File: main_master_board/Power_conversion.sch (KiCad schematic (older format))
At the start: 60 parts

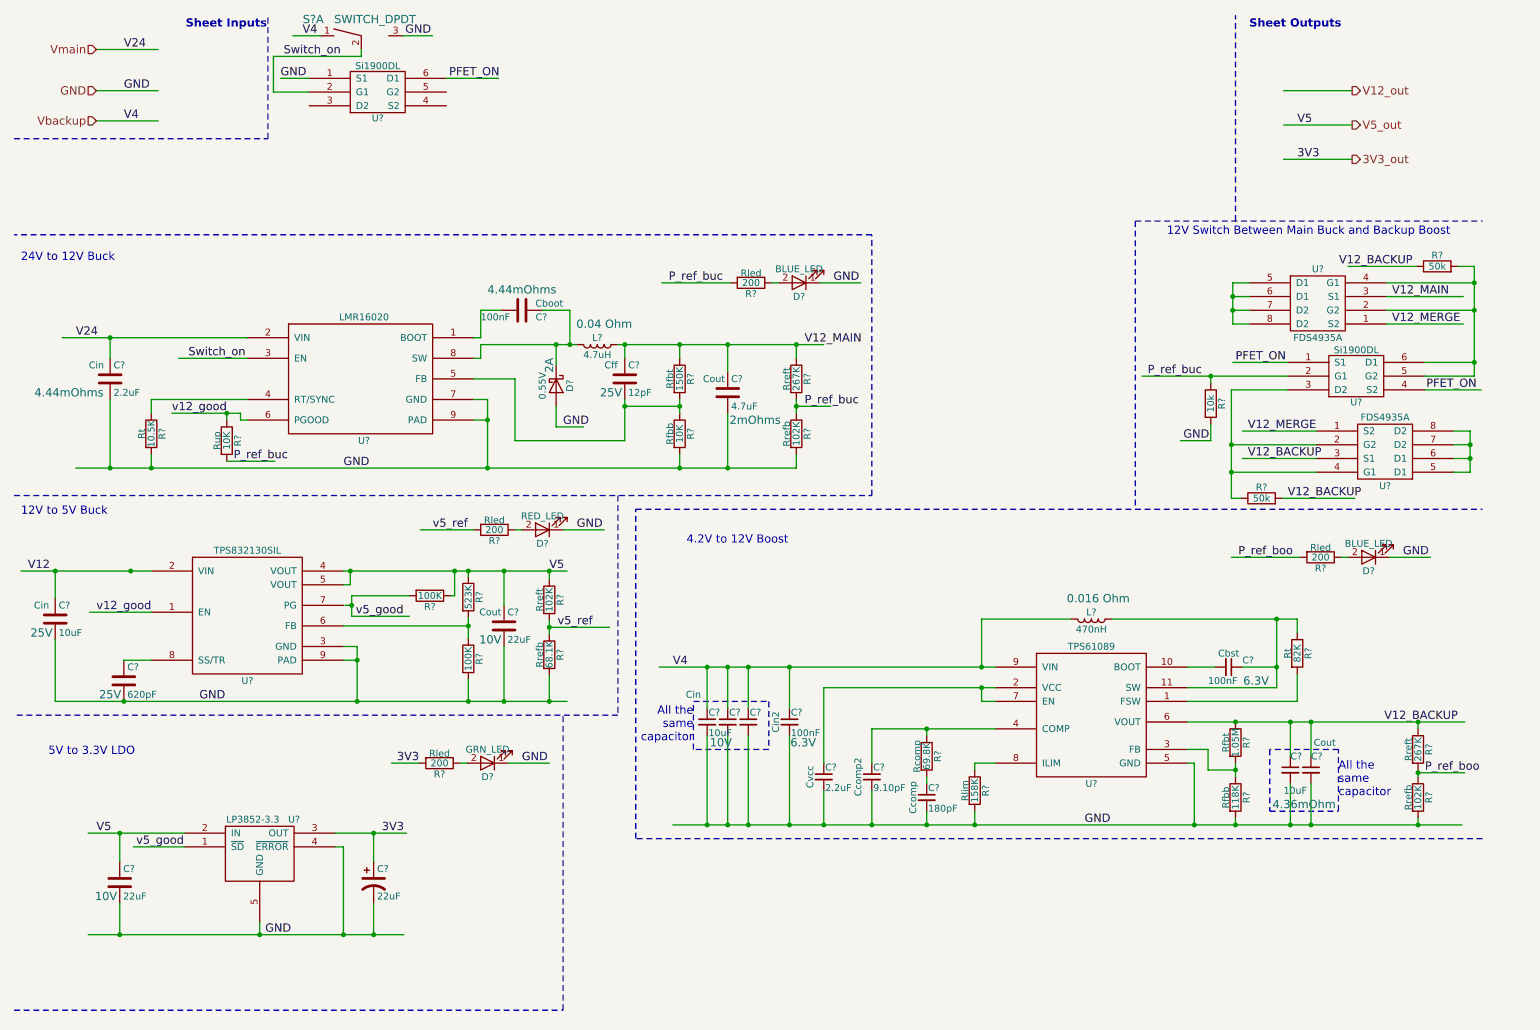
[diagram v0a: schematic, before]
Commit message: Added lots of things. current/voltage monitoring. and other stuff
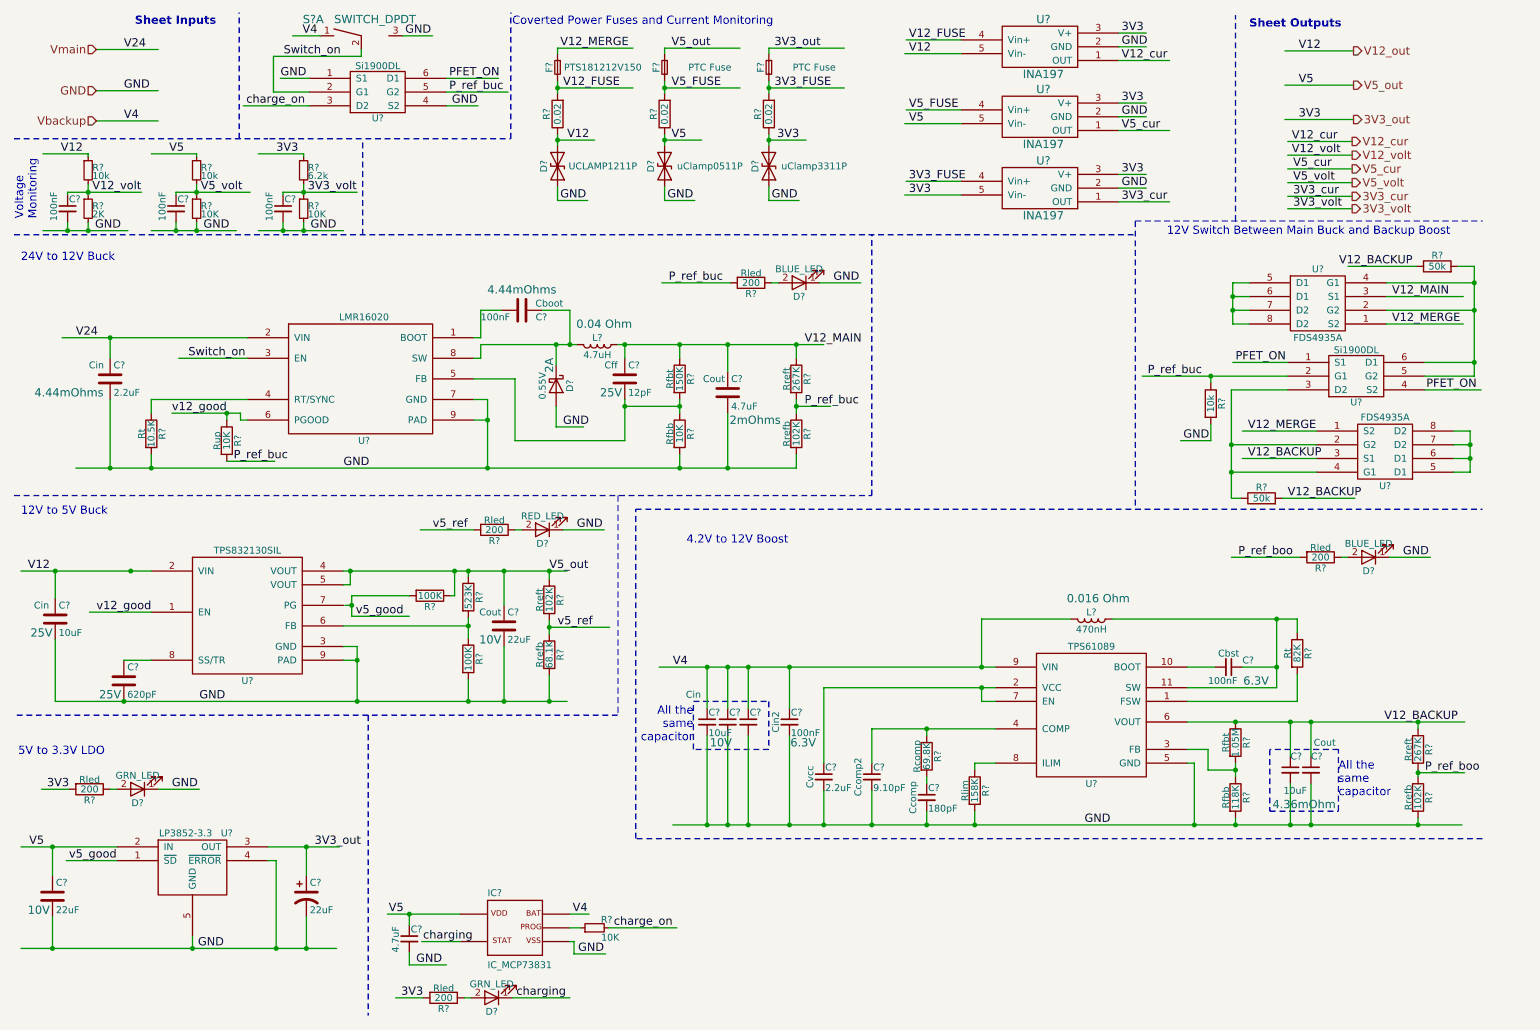
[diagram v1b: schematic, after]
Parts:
- added C? (x3): 100nF, symbol C_Small
- added C?: 4.7uF, symbol C_Small
- added D?: UCLAMP1211P, symbol D_TVS
- added D?: uClamp0511P, symbol D_TVS
- added D?: uClamp3311P, symbol D_TVS
- added D?: GRN_LED, 754-1126-1-ND, symbol LED-RESCUE-main_master_board
- added F?: PTS181212V150, symbol Fuse_Small
- added F? (x2): PTC Fuse, symbol Fuse_Small
- added IC?: IC_MCP73831, dp_devices-SOT-23-5, symbol IC_MCP73831
- added R? (x3): 0.02, symbol R
- added R? (x2): 10k, symbol R_Small
- added R?: 2K, symbol R_Small
- added R? (x3): 10K, symbol R_Small
- added R?: 6.2k, symbol R_Small
- added R?: 200, Rled, symbol R
- added U? (x3): INA197, symbol INA197
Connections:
- net labels added: 3V3_FUSE, 3V3_cur, 3V3_volt, V12_FUSE, V12_cur, V12_volt, V5_FUSE, V5_cur, V5_volt, charge_on, charging
- wire segments 191 -> 277
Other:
- note added: "Coverted Power Fuses and Current Monitoring"
- note added: "Voltage \nMonitoring"
- moved on the sheet: C?, D?, R?, U?
